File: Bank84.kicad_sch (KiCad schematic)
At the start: 1 part, among them U1 XCKU5P-FFVB676

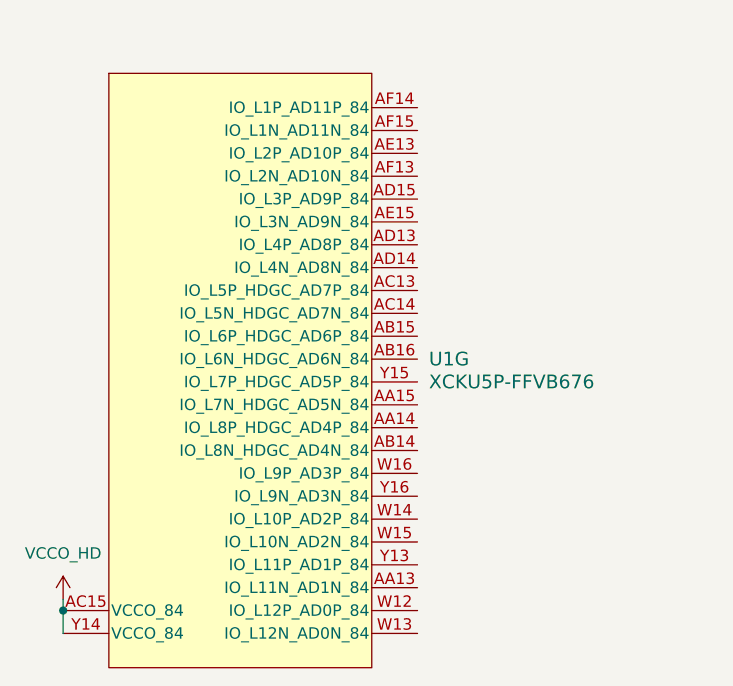
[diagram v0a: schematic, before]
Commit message: finishing schematic
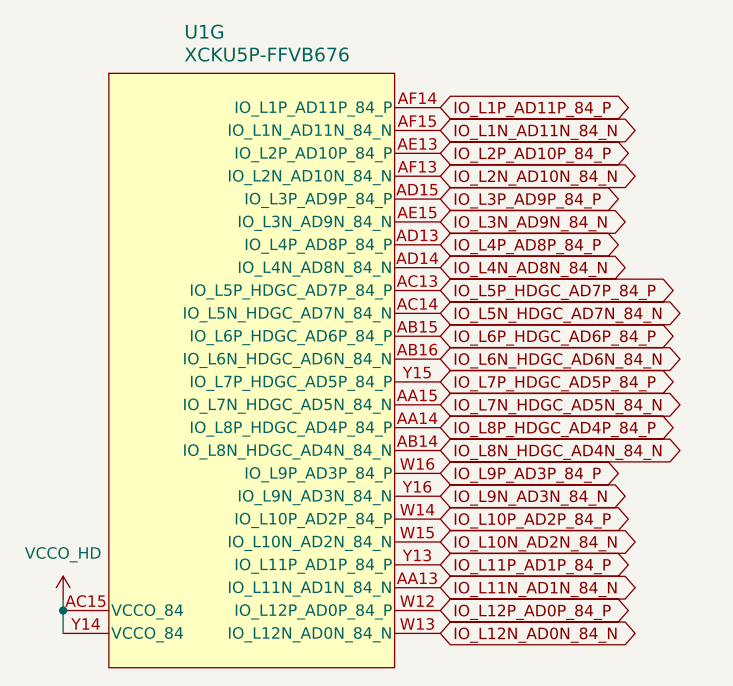
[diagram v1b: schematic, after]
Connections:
- net IO_L11N_AD1N_84_N: now reaches U1.AA13 (IO_L11N_AD1N_84_N)
- net IO_L8P_HDGC_AD4P_84_P: now reaches U1.AA14 (IO_L8P_HDGC_AD4P_84_P)
- net IO_L7N_HDGC_AD5N_84_N: now reaches U1.AA15 (IO_L7N_HDGC_AD5N_84_N)
- net IO_L8N_HDGC_AD4N_84_N: now reaches U1.AB14 (IO_L8N_HDGC_AD4N_84_N)
- net IO_L6P_HDGC_AD6P_84_P: now reaches U1.AB15 (IO_L6P_HDGC_AD6P_84_P)
- net IO_L6N_HDGC_AD6N_84_N: now reaches U1.AB16 (IO_L6N_HDGC_AD6N_84_N)
- net IO_L5P_HDGC_AD7P_84_P: now reaches U1.AC13 (IO_L5P_HDGC_AD7P_84_P)
- net IO_L5N_HDGC_AD7N_84_N: now reaches U1.AC14 (IO_L5N_HDGC_AD7N_84_N)
- net IO_L4P_AD8P_84_P: now reaches U1.AD13 (IO_L4P_AD8P_84_P)
- net IO_L4N_AD8N_84_N: now reaches U1.AD14 (IO_L4N_AD8N_84_N)
- net IO_L3P_AD9P_84_P: now reaches U1.AD15 (IO_L3P_AD9P_84_P)
- net IO_L2P_AD10P_84_P: now reaches U1.AE13 (IO_L2P_AD10P_84_P)
- net IO_L3N_AD9N_84_N: now reaches U1.AE15 (IO_L3N_AD9N_84_N)
- net IO_L2N_AD10N_84_N: now reaches U1.AF13 (IO_L2N_AD10N_84_N)
- net IO_L1P_AD11P_84_P: now reaches U1.AF14 (IO_L1P_AD11P_84_P)
- net IO_L1N_AD11N_84_N: now reaches U1.AF15 (IO_L1N_AD11N_84_N)
- net IO_L12P_AD0P_84_P: now reaches U1.W12 (IO_L12P_AD0P_84_P)
- net IO_L12N_AD0N_84_N: now reaches U1.W13 (IO_L12N_AD0N_84_N)
- net IO_L10P_AD2P_84_P: now reaches U1.W14 (IO_L10P_AD2P_84_P)
- net IO_L10N_AD2N_84_N: now reaches U1.W15 (IO_L10N_AD2N_84_N)
- net IO_L9P_AD3P_84_P: now reaches U1.W16 (IO_L9P_AD3P_84_P)
- net IO_L11P_AD1P_84_P: now reaches U1.Y13 (IO_L11P_AD1P_84_P)
- net IO_L7P_HDGC_AD5P_84_P: now reaches U1.Y15 (IO_L7P_HDGC_AD5P_84_P)
- net IO_L9N_AD3N_84_N: now reaches U1.Y16 (IO_L9N_AD3N_84_N)
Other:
- moved on the sheet: U1G
